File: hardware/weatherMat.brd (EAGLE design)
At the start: 162.7 x 112.7 mm, 29 parts, among them IC1 MCP3008, IC2 LM2596S, J1 MAGJACK, J2 RASPBERRYPI-40-PIN-GPIOJIM, J3 Air Digitals, J4 Soil Temp, J5 Air Analogs, J6 RJ11, J7 RJ11, U1 MAGJACK-POE

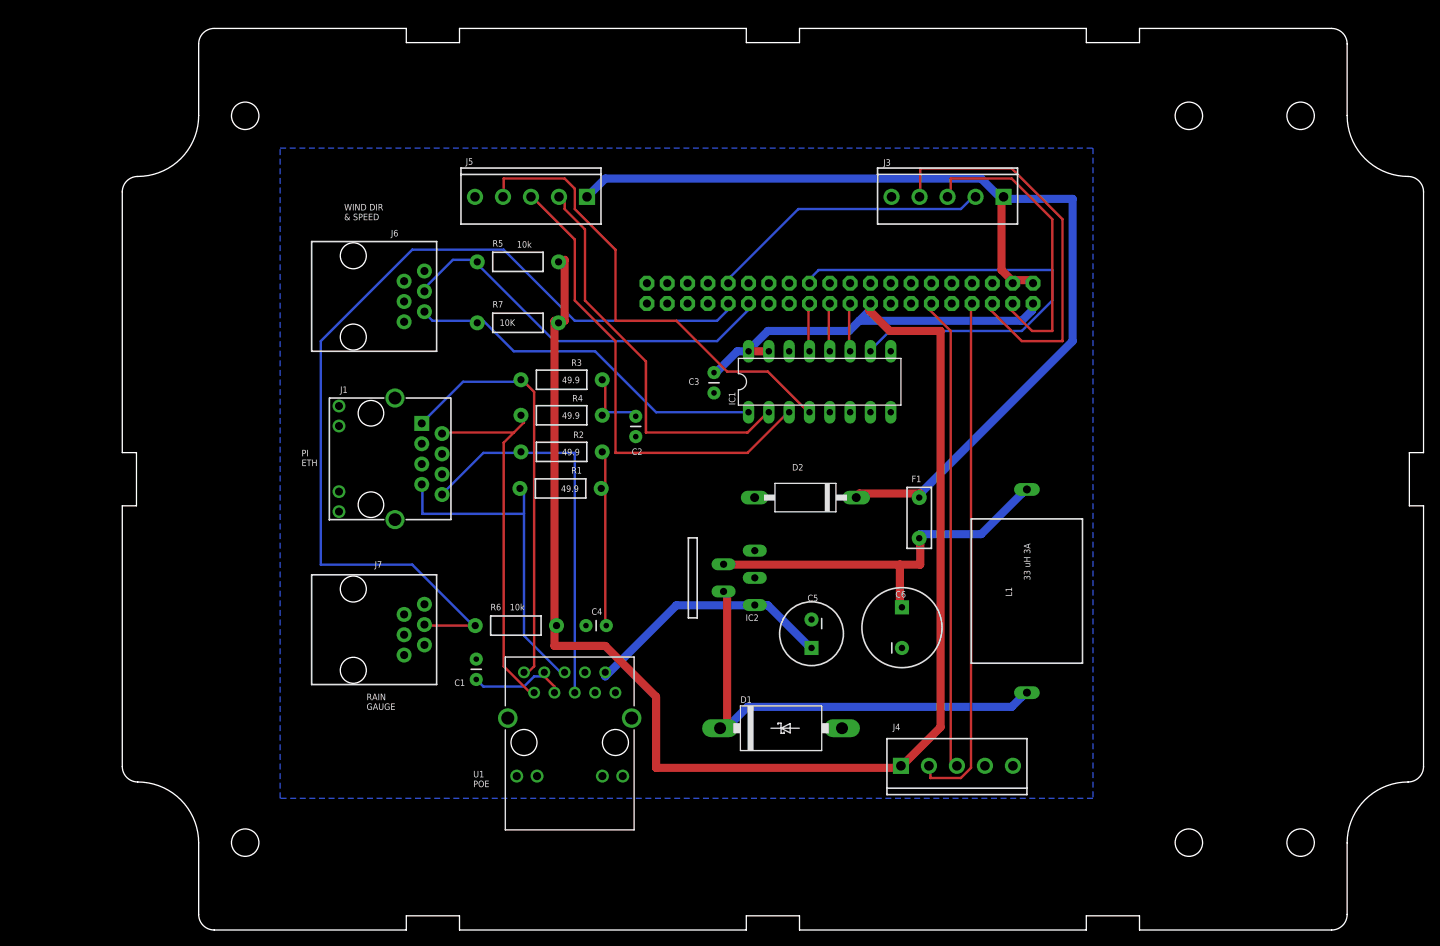
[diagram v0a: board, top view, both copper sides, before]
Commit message: Update
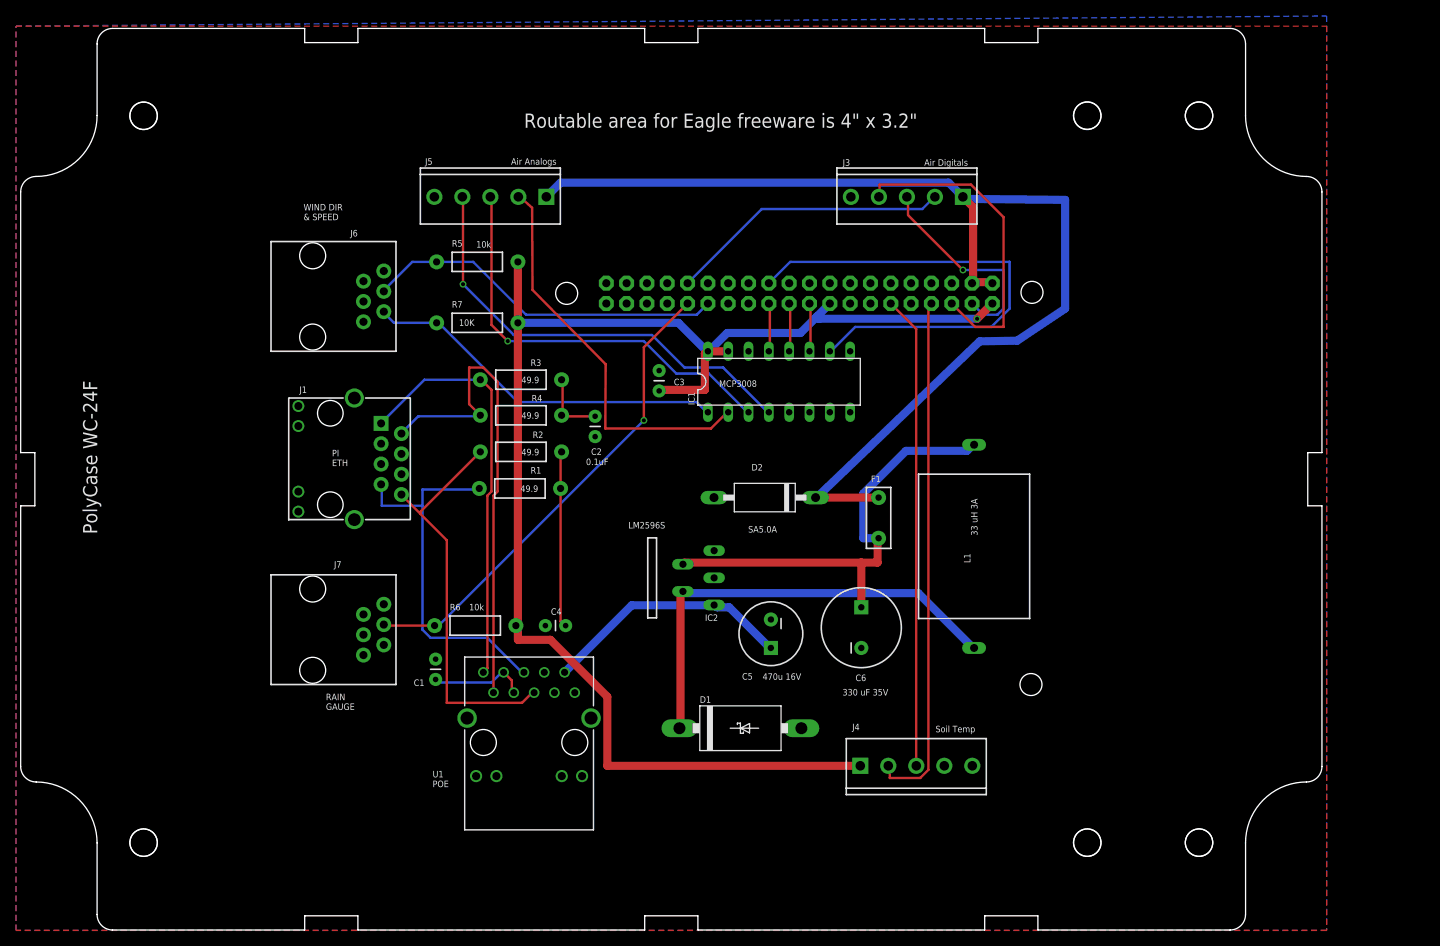
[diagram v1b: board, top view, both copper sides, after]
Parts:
- moved U$1 29.2 mm to (186.7, 42.4)
- moved U$2 12.7 mm to (-32.6, -16.0)
- moved L1 8.65 mm to (86.7, 31.5)
- moved C3 7.23 mm to (47.4, 50.9), turned to 90 degrees
- moved J3 5.08 mm to (85.3, 75.2)
- moved C2 5.08 mm to (39.4, 47.8)
- moved C4 5.08 mm to (35.7, 21.6)
- moved C5 5.08 mm to (61.3, 20.6)
- moved D2 5.08 mm to (60.6, 37.6)
- moved R2 5.08 mm to (30.1, 43.3)
- moved R3 5.08 mm to (30.1, 52.3)
- moved R4 5.08 mm to (30.1, 47.9)
- moved U1 5.08 mm to (31.1, 6.86)
- moved J1 5.08 mm to (-4.83, 50.0)
- moved J6 5.08 mm to (4.06, 62.7)
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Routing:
- net GP6: track 117.9 -> 60.1 mm, vias 0 -> 1
- net +3V3: track 222.5 -> 180.9 mm, vias 0 -> 1
- net N$6: track 47.4 -> 60.7 mm
- net N$15: track 38.8 -> 26.9 mm, vias 0 -> 1
- net N$16: track 51.1 -> 40.2 mm
- net +5V: track 131.8 -> 142.1 mm
- net N$14: track 49.5 -> 57.0 mm
- net N$18: track 60.3 -> 52.8 mm, vias 0 -> 1
- net N$3: track 42.9 -> 47.4 mm
- net GP5: track 49.8 -> 45.4 mm
- net N$19: track 59.8 -> 55.9 mm, vias 0 -> 1
- net N$2: track 14.5 -> 12.4 mm
- net N$1: track 58.2 -> 56.6 mm
- net N$5: track 53.5 -> 52.3 mm
- net N$12: track 60.8 -> 61.7 mm
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- added copper zone on layer 1, net GND
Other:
- board text added: "PolyCase WC-24F"
- board text added: "Routable area for Eagle freeware is 4" x 3.2""

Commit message: Update
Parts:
- removed U$1: (no value), Jims:PIOUTLINE
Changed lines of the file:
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@@
 </element>
 <element name="U$2" library="Jims" package="WC-24F" value="" x="-32.639" y="-16.002"/>
-<element name="U$1" library="Jims" package="PIOUTLINE" value="" x="186.69" y="42.418"/>
 <element name="C1" library="SparkFun-Capacitors" package="CAP-PTH-SMALL" value="0.1uF" x="19.431" y="14.859" smashed="yes" rot="R90">
 <attribute name="NAME" x="18.034" y="14.859" size="0.8128" layer="25" font="vector" ratio="12" rot="R180"/>
